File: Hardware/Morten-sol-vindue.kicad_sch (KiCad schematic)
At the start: 26 parts, among them J1 Conn_01x04, J2 CUI_PJ-079BH, J3 SJ-43514-SMT, J4 AudioJack4, U3 ATtiny412-SS, U4 LM358, U5 SHT4x

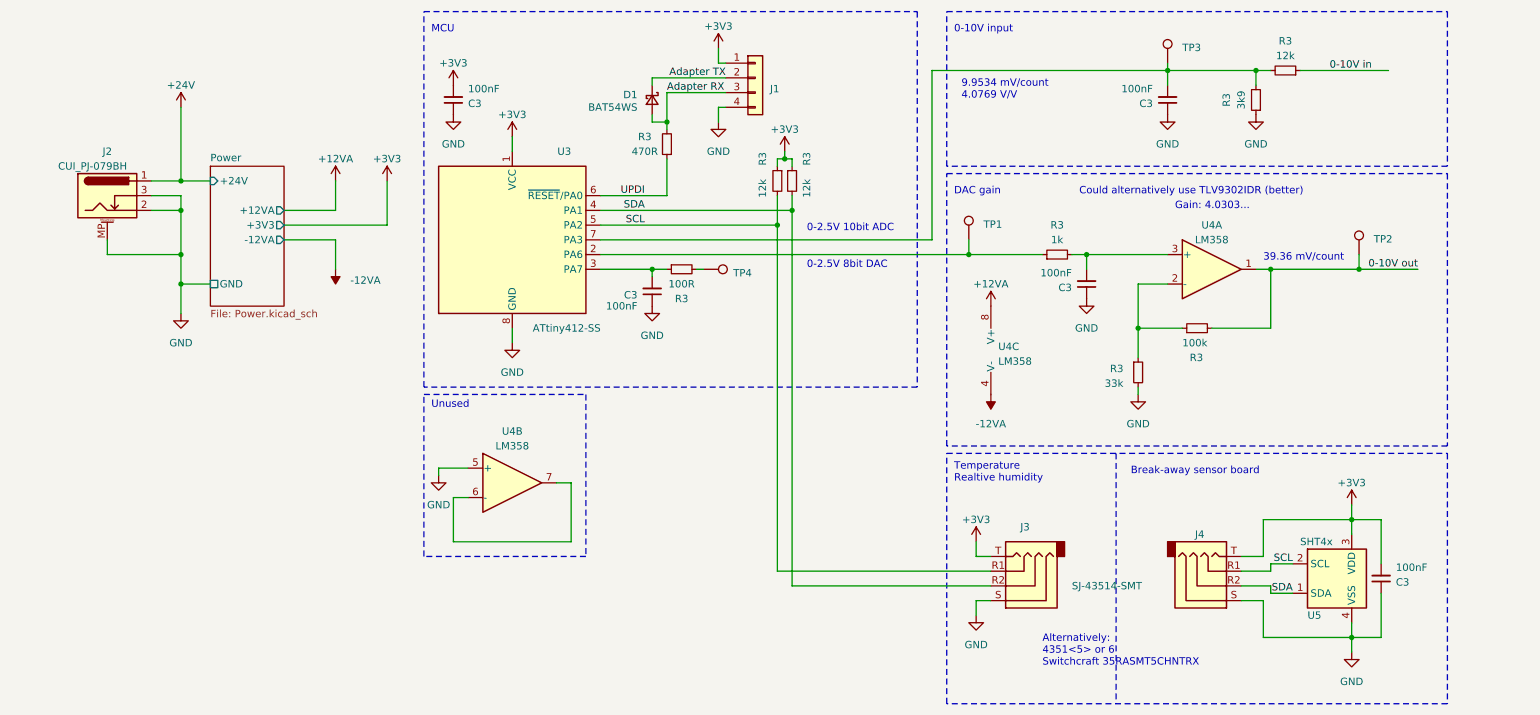
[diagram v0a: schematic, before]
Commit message: Initial layout
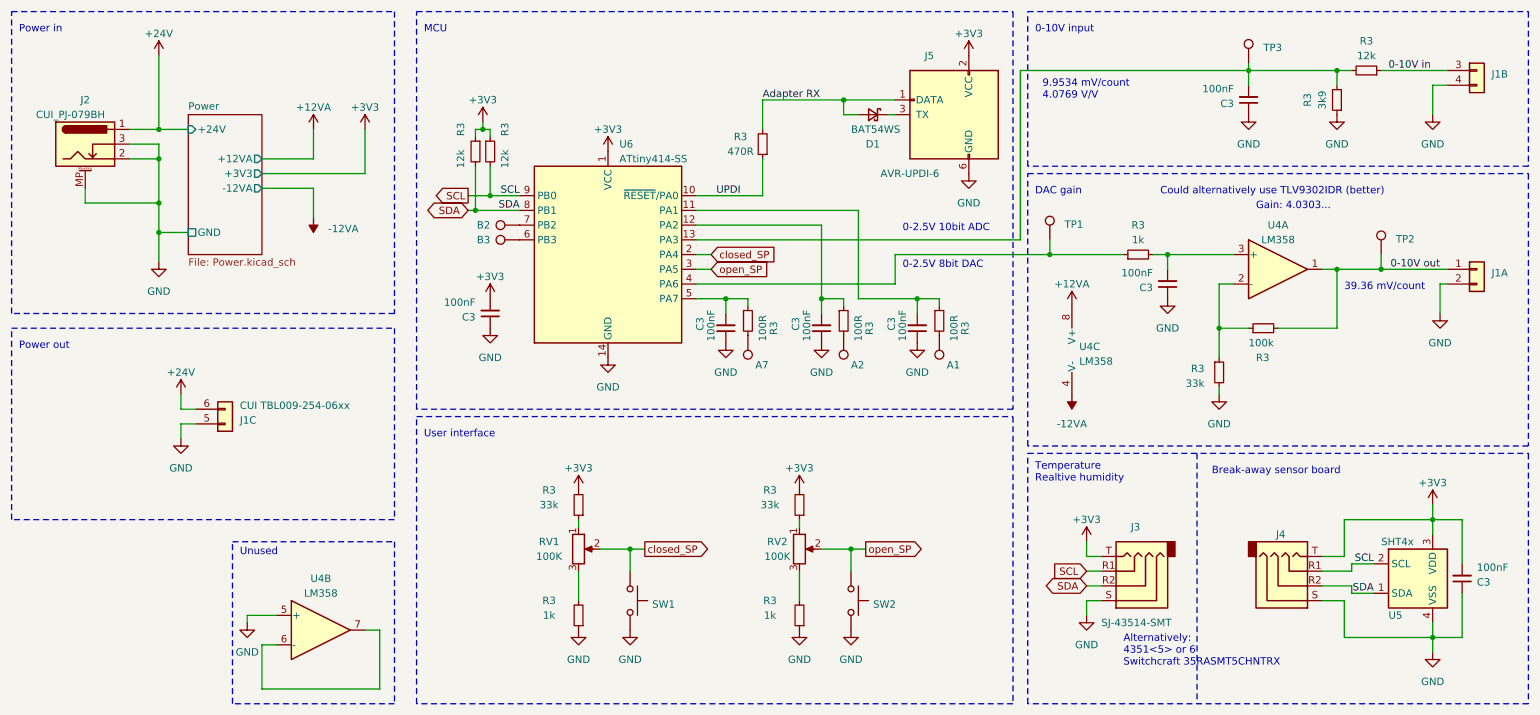
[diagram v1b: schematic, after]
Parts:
- removed J1: Conn_01x04, Connector_PinHeader_2.54mm:PinHeader_1x04_P2.54mm_Vertical, symbol Connector_Generic:Conn_01x04
- removed U3: ATtiny412-SS, Package_SO:SOIC-8_3.9x4.9mm_P1.27mm, symbol MCU_Microchip_ATtiny:ATtiny412-SS
- added A1, A2, B2, B3: PA7, TestPoint:TestPoint_Pad_D1.0mm, symbol Connector:TestPoint
- added C3 (x2): 100nF, Capacitor_SMD:C_0603_1608Metric_Pad1.08x0.95mm_HandSolder, symbol Device:C_Small
- added J1: CUI TBL009-254-06xx, TerminalBlock_Phoenix:TerminalBlock_Phoenix_PTSM-0,5-6-2.5-H-THR_1x06_P2.50mm_Horizontal, symbol Connector_Generic:Conn_01x02
- added J5: AVR-UPDI-6, Connector:Tag-Connect_TC2030-IDC-FP_2x03_P1.27mm_Vertical, symbol Connector:AVR-UPDI-6
- added R3 (x2): 33k, Resistor_SMD:R_0603_1608Metric_Pad0.98x0.95mm_HandSolder, symbol Device:R_Small
- added R3 (x2): 100R, Resistor_SMD:R_0603_1608Metric_Pad0.98x0.95mm_HandSolder, symbol Device:R_Small
- added R3 (x2): 1k, Resistor_SMD:R_0603_1608Metric_Pad0.98x0.95mm_HandSolder, symbol Device:R_Small
- added RV1, RV2: 100K, Potentiometer_THT:Potentiometer_Bourns_PTV09A-1_Single_Vertical, symbol Device:R_Potentiometer
- added SW1, SW2: SW_Push, Button_Switch_SMD:SW_Push_1P1T_NO_6x6mm_H9.5mm, symbol Switch:SW_Push
- added U6: ATtiny414-SS, Package_SO:SOIC-14_3.9x8.7mm_P1.27mm, symbol MCU_Microchip_ATtiny:ATtiny414-SS
- renumbered TP4 to A7
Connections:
- net +24V: now also J1.6 (Pin_6)
- net +3V3: now also J5.2 (VCC), R3.2, R3.2, U6.1 (VCC)
- net 0-10V in: now also J1.3 (Pin_3)
- net 0-10V out: now also J1.1 (Pin_1)
- net Adapter RX: now also J5.1 (DATA)
- net GND: now also C3.1, C3.1, J1.2 (Pin_2), J1.4 (Pin_4), J1.5 (Pin_5), J5.6 (GND), R3.1, R3.1, SW1.2, SW2.2, U6.14 (GND)
- net SCL: now also R3.2, U6.9 (PB0); no longer R3.2
- net SDA: now also R3.2, U6.8 (PB1); no longer R3.2
- net UPDI: now also U6.10 (~{RESET}/PA0)
- net at R3.1, TP1.1: now also U6.4 (PA6)
- net at C3.2, R3.1: now also U6.5 (PA7)
- net at C3.2, R3.2, R3.2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: now also U6.13 (PA3)
- net Adapter TX: no longer names the net of D1.1 (K)
- net Adapter TX: now also J5.3 (TX)
- new net: R3.1, RV2.1
- new net: C3.2, R3.1, U6.12 (PA2)
- new net: C3.2, R3.1, U6.11 (PA1)
- new net: A1.1, R3.2
- new net: A2.1, R3.2
- new net: R3.1, RV1.1
- new net: R3.2, RV1.3
- new net: R3.2, RV2.3
- new net: B2.1, U6.7 (PB2)
- new net: B3.1, U6.6 (PB3)
- new net closed_SP: RV1.2, SW1.1, U6.2 (PA4)
- new net open_SP: RV2.2, SW2.1, U6.3 (PA5)
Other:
- note added: "Power in"
- note added: "Power out"
- note added: "User interface"
- moved on the sheet: A7, C3, D1, J2, J3, J4, R3, TP1, TP2, TP3, U4A, U4B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

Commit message: Re-layout
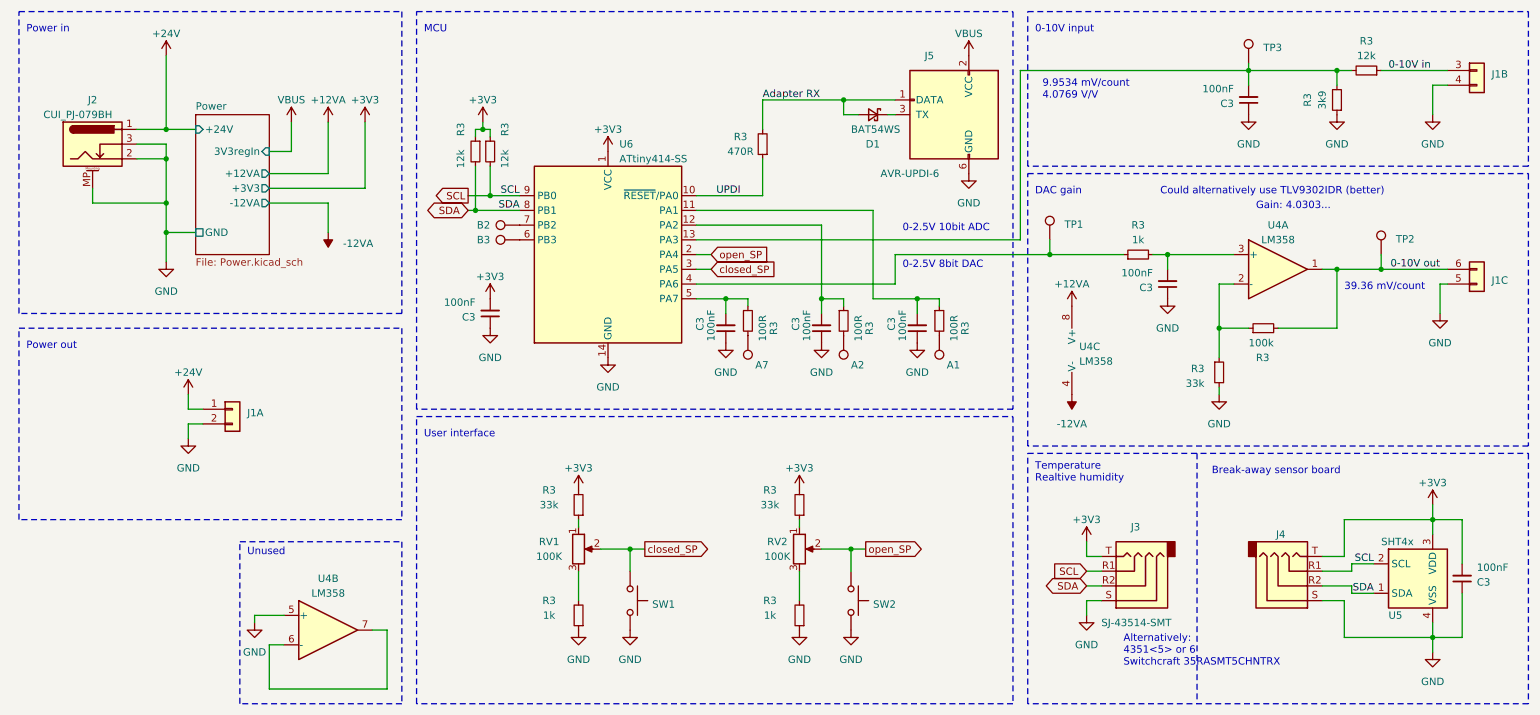
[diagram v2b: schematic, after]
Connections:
- net +24V: now also J1.1 (Pin_1); no longer J1.6 (Pin_6)
- net +3V3: no longer J5.2 (VCC)
- net 0-10V out: now also J1.6 (Pin_6); no longer J1.1 (Pin_1)
- net closed_SP: now also U6.3 (PA5); no longer U6.2 (PA4)
- net open_SP: now also U6.2 (PA4); no longer U6.3 (PA5)
- new net VBUS: J5.2 (VCC)
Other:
- sheet Power ports: added 3V3regIn; removed none
- moved on the sheet: J1A, J1C, J2, U4B
